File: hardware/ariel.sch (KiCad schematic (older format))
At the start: 19 parts, among them SW1 SW_Push, U1 74HC595, U2 Si7020-A20, U3 WeMos_Battery_Shield, U4 WeMos_D1_mini

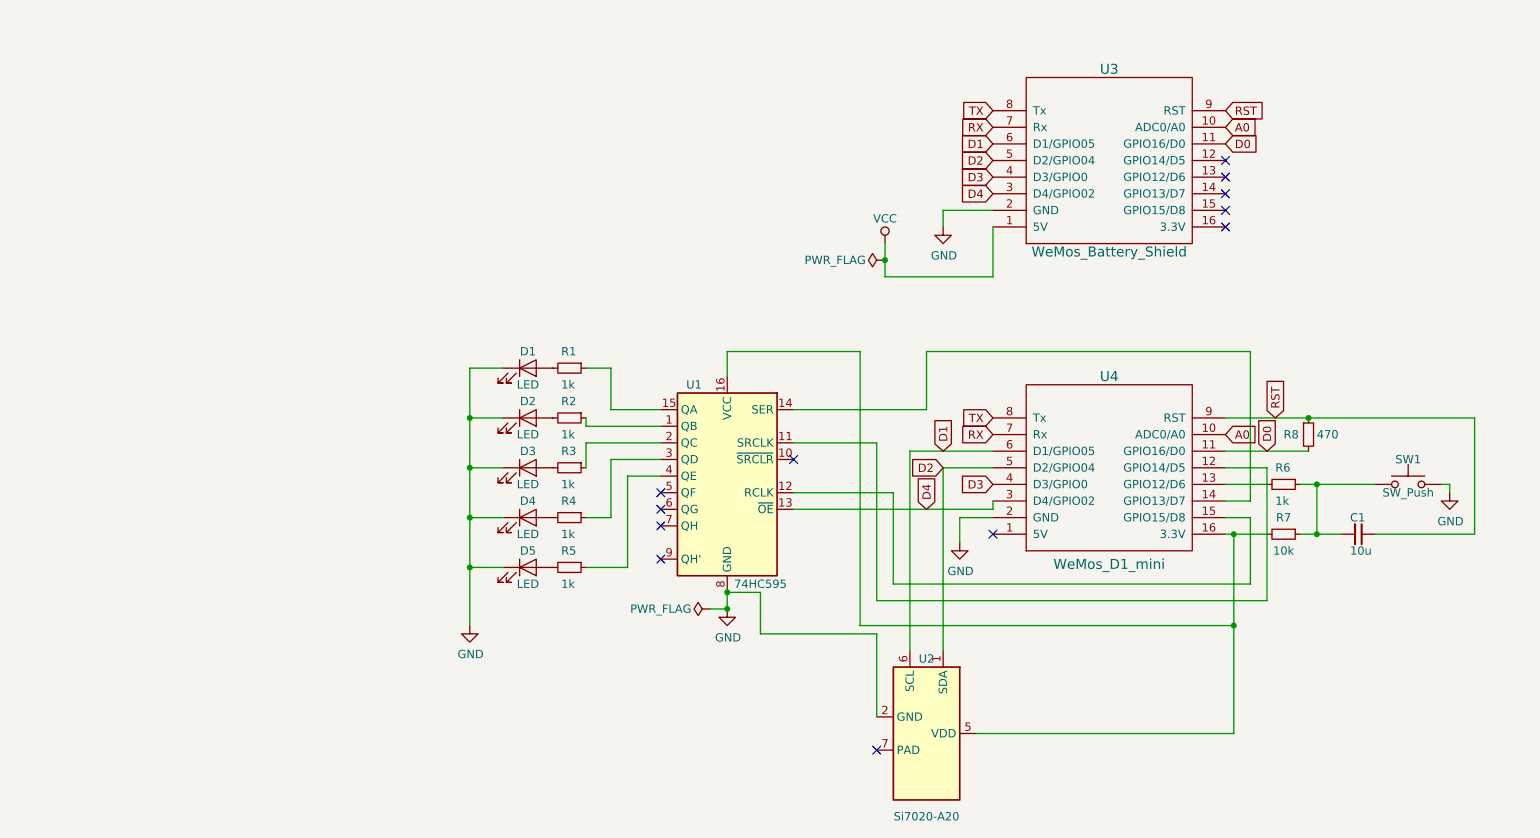
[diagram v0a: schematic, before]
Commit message: Cleanup schematic and pass ERC
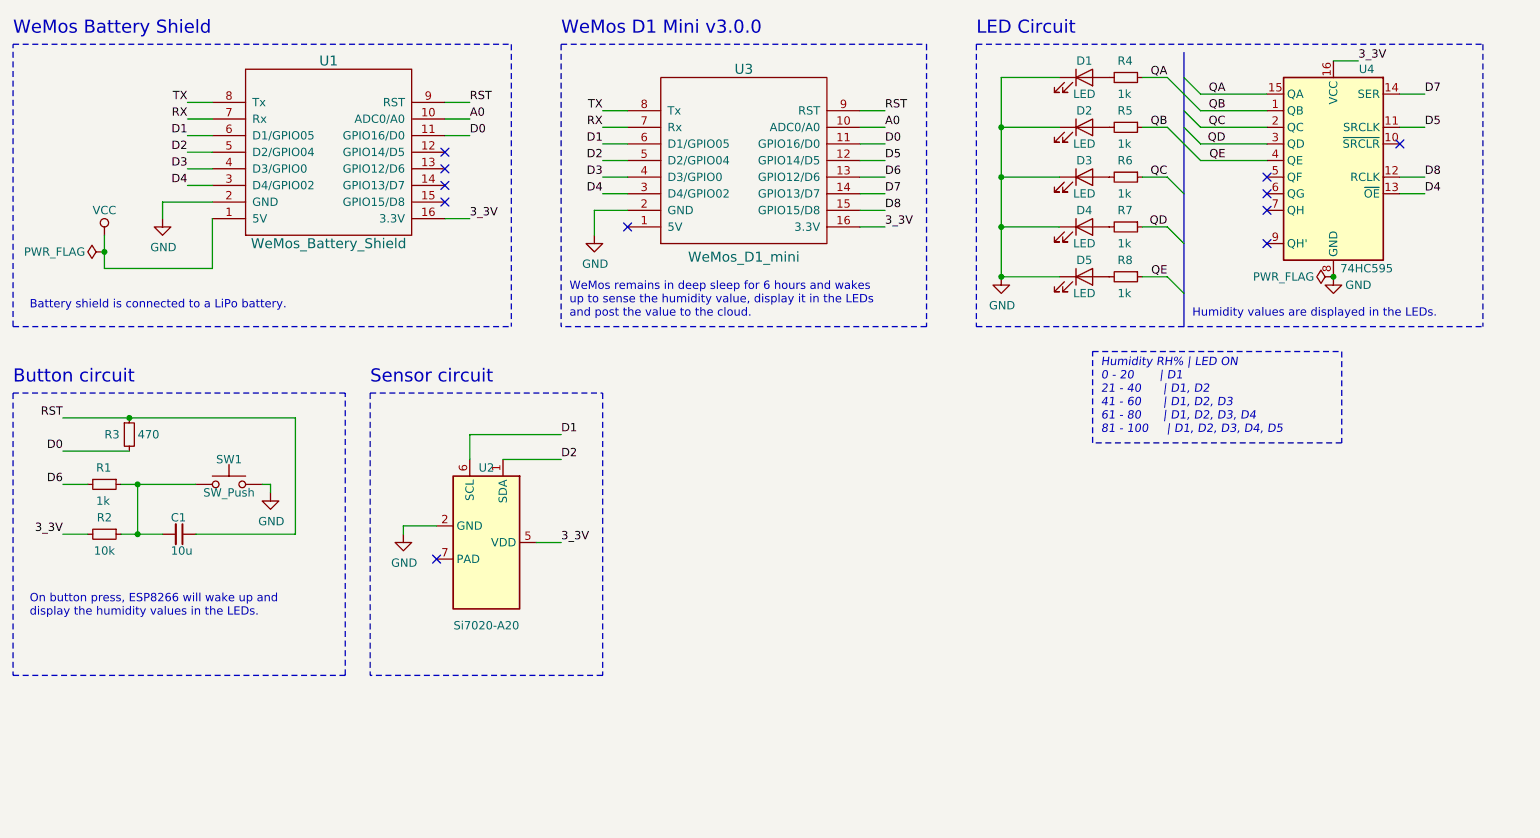
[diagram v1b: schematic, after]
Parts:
- renumbered R6 to R1, R7 to R2, R8 to R3, R1 to R4, R2 to R5, R3 to R6, R4 to R7, R5 to R8, U3 to U1, U4 to U3, U1 to U4
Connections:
- net QB: now reaches R5.1, U4.1 (QB)
- net D5: now reaches U3.12 (GPIO14/D5), U4.11 (SRCLK)
- net D8: now reaches U3.15 (GPIO15/D8), U4.12 (RCLK)
- net D7: now reaches U3.14 (GPIO13/D7), U4.14 (SER)
- net QA: now reaches R4.1, U4.15 (QA)
- net 3_3V: now reaches R2.2, U2.5 (VDD), U3.16 (3.3V), U4.16 (VCC)
- net 3_3V: now also U1.16 (3.3V)
- net QC: now reaches R6.1, U4.2 (QC)
- net QD: now reaches R7.1, U4.3 (QD)
- net QE: now reaches R8.1, U4.4 (QE)
- net D6: now reaches R1.2, U3.13 (GPIO12/D6)
- no-connect marks 12 -> 11
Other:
- note added: "Battery shield is connected to a LiPo battery."
- note added: "Button circuit"
- note added: "Humidity RH% | LED ON\n0 - 20 | D1\n21 - 40 | D1, D2\n41 - 60 | D1, D2, D3\n61 - 80 | D1, D2, D3, D4\n81 - 100 | D1, D2, D3, D4, D5"
- note added: "Humidity values are displayed in the LEDs."
- note added: "LED Circuit"
- note added: "On button press, ESP8266 will wake up and \ndisplay the humidity values in the LEDs."
- note added: "Sensor circuit"
- note added: "WeMos Battery Shield"
- note added: "WeMos D1 Mini v3.0.0"
- note added: "WeMos remains in deep sleep for 6 hours and wakes \nup to sense the humidity value, display it in the LEDs \nand post the value to the cloud."
- moved on the sheet: C1, D1, D2, D3, D4, D5, R1, R2, R3, R4, R5, R6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
